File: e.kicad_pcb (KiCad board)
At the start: 2 copper layers, 80 x 58.5 mm, 9 parts, among them SW1 usr, SW2 rst, U1 Display_ST7789, U2 MAX98357A

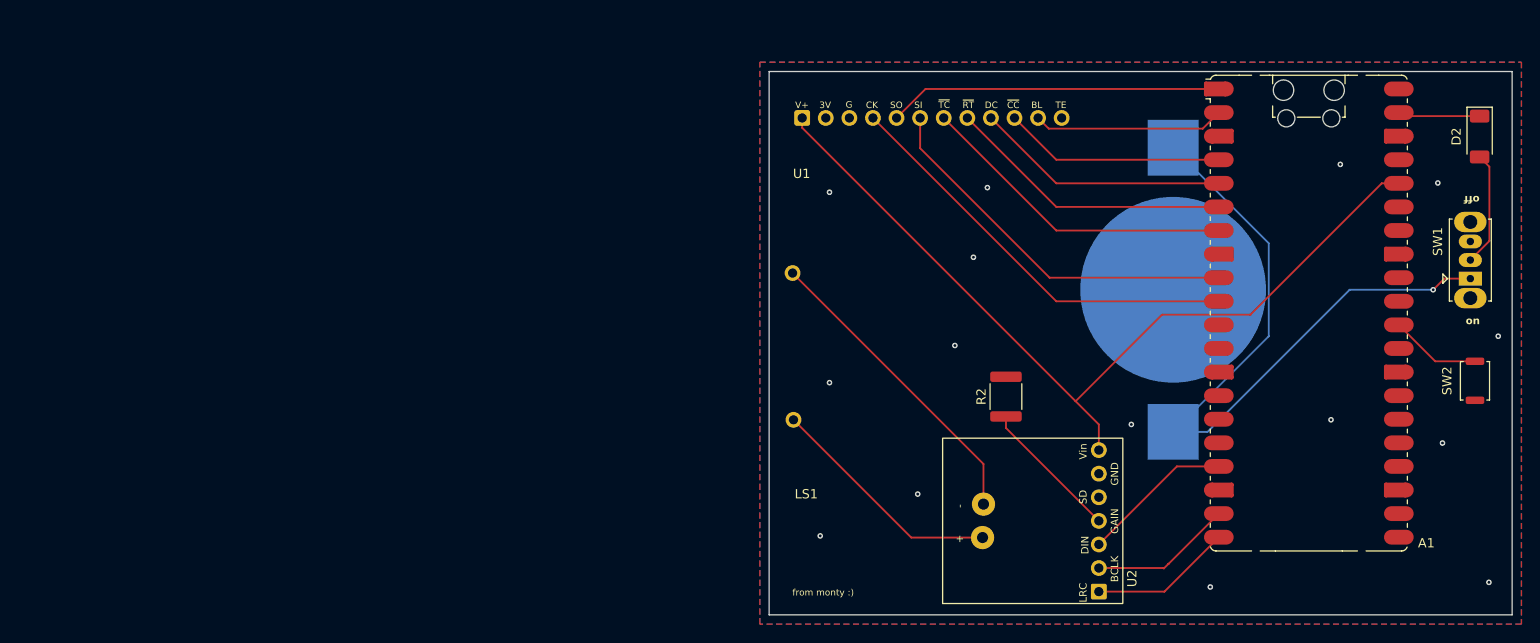
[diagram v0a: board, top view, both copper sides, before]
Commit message: edited page stuff
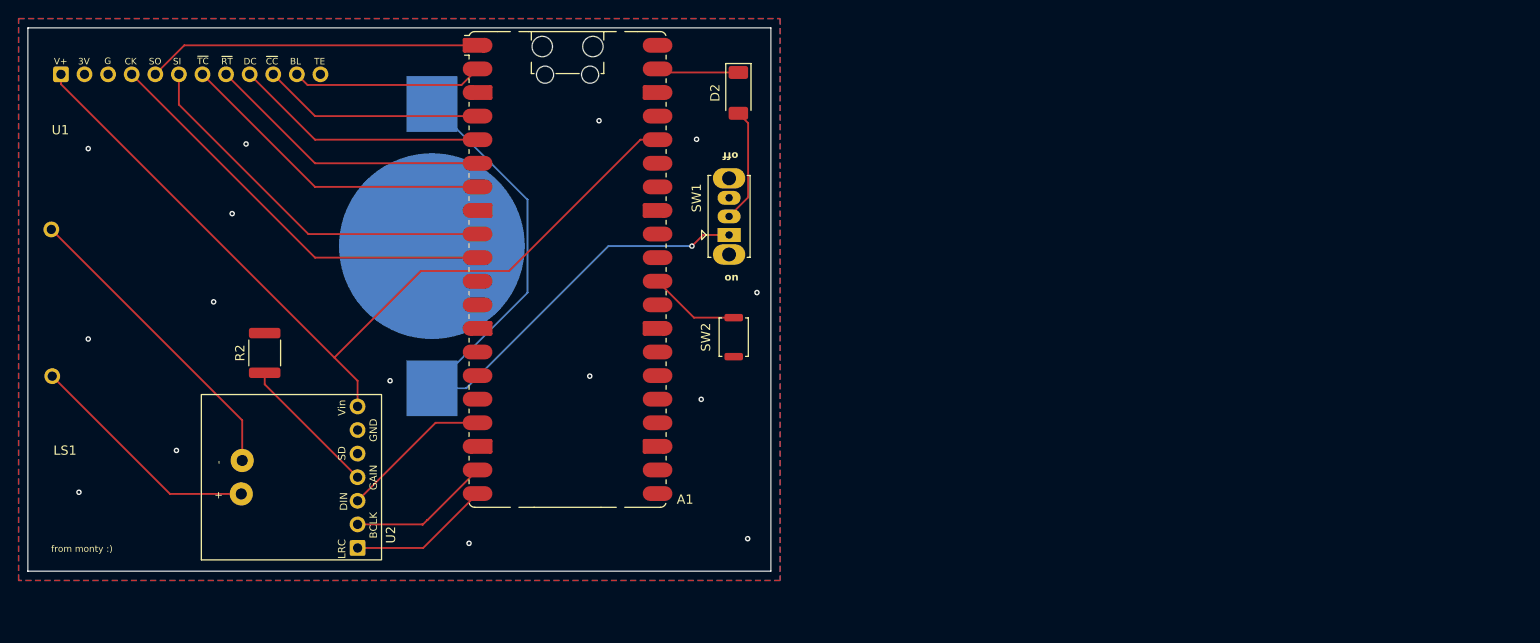
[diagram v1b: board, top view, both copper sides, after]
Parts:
- moved A1 79.9 mm to (162.8, 100.3)
- moved BT1 79.9 mm to (148.2, 97.8)
- moved D2 79.9 mm to (181.2, 81.3)
- moved LS1 79.9 mm to (106.7, 103.7)
- moved R2 79.9 mm to (130.2, 109.3)
- moved SW1 79.9 mm to (180.2, 96.6)
- moved SW2 79.9 mm to (180.7, 107.6)
- moved U1 79.9 mm to (122.2, 63.1)
- moved U2 79.9 mm to (133.3, 122.7)
